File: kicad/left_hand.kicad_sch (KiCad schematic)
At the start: 29 parts, among them SW10 Gateron_ks_27, SW11 Gateron_ks_27, SW12 Gateron_ks_27, SW13 Gateron_ks_27, SW14 Gateron_ks_27, SW15 Gateron_ks_27, SW16 Gateron_ks_27, SW17 Gateron_ks_27, SW18 Gateron_ks_27, SW19 Gateron_ks_27, SW20 Gateron_ks_27, SW21 Gateron_ks_27, SW22 Gateron_ks_27, SW23 Gateron_ks_27, SW24 Gateron_ks_27, SW25 Gateron_ks_27, SW26 Gateron_ks_27, SW27 Gateron_ks_27, SW28 Gateron_ks_27, SW29 Gateron_ks_27, SW30 Gateron_ks_27, SW31 Gateron_ks_27, SW32 Gateron_ks_27, SW33 Gateron_ks_27, SW6 Gateron_ks_27, SW7 Gateron_ks_27, SW8 Gateron_ks_27, SW9 Gateron_ks_27, U2 74HC595

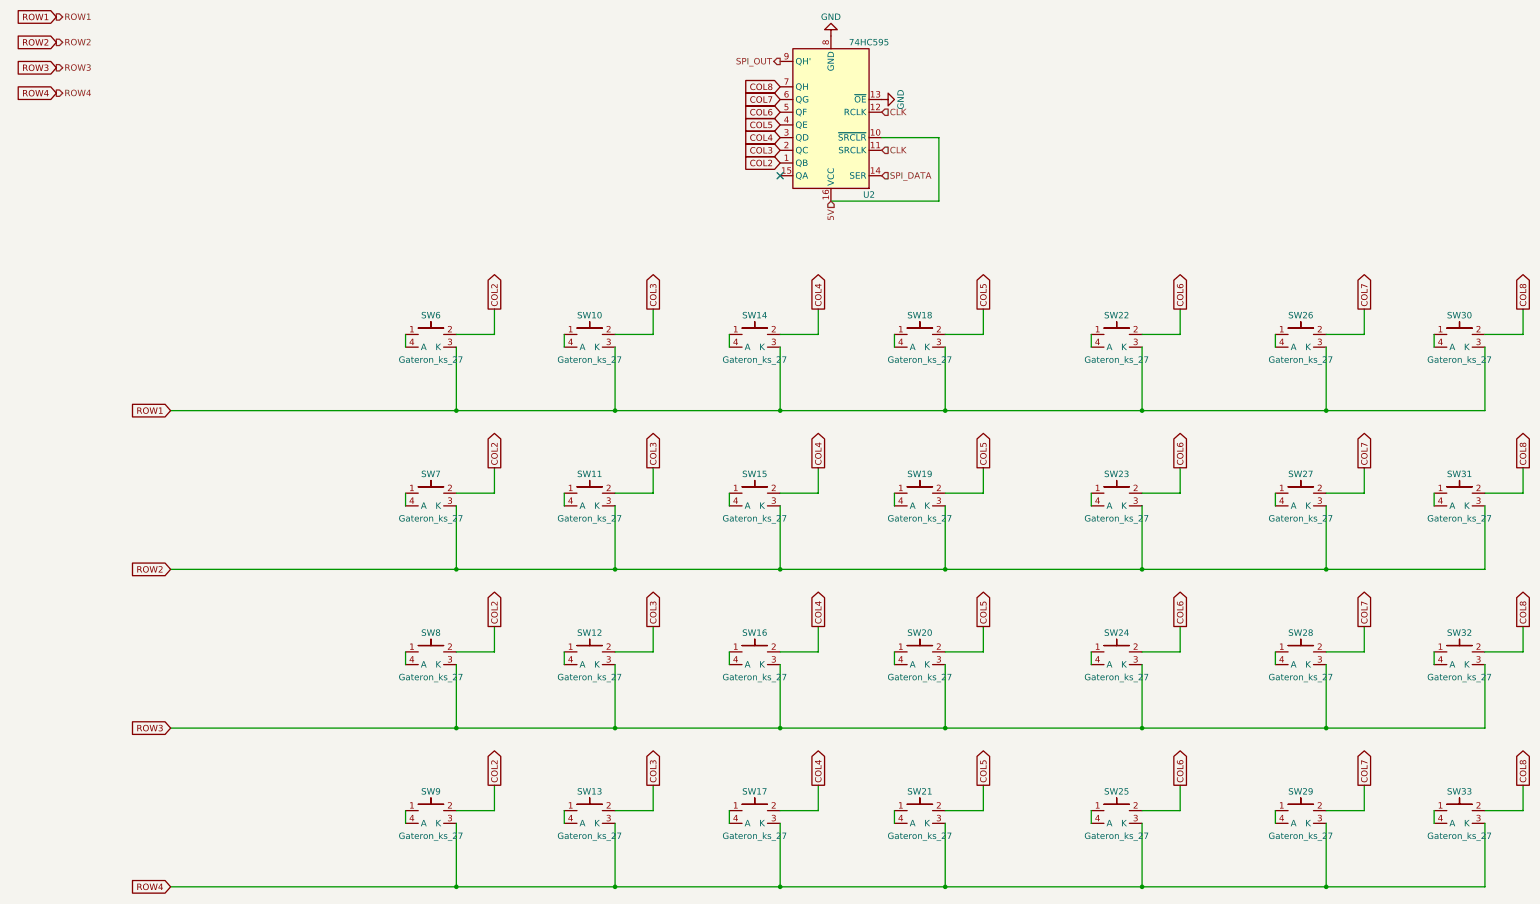
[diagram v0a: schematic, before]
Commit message: Last update
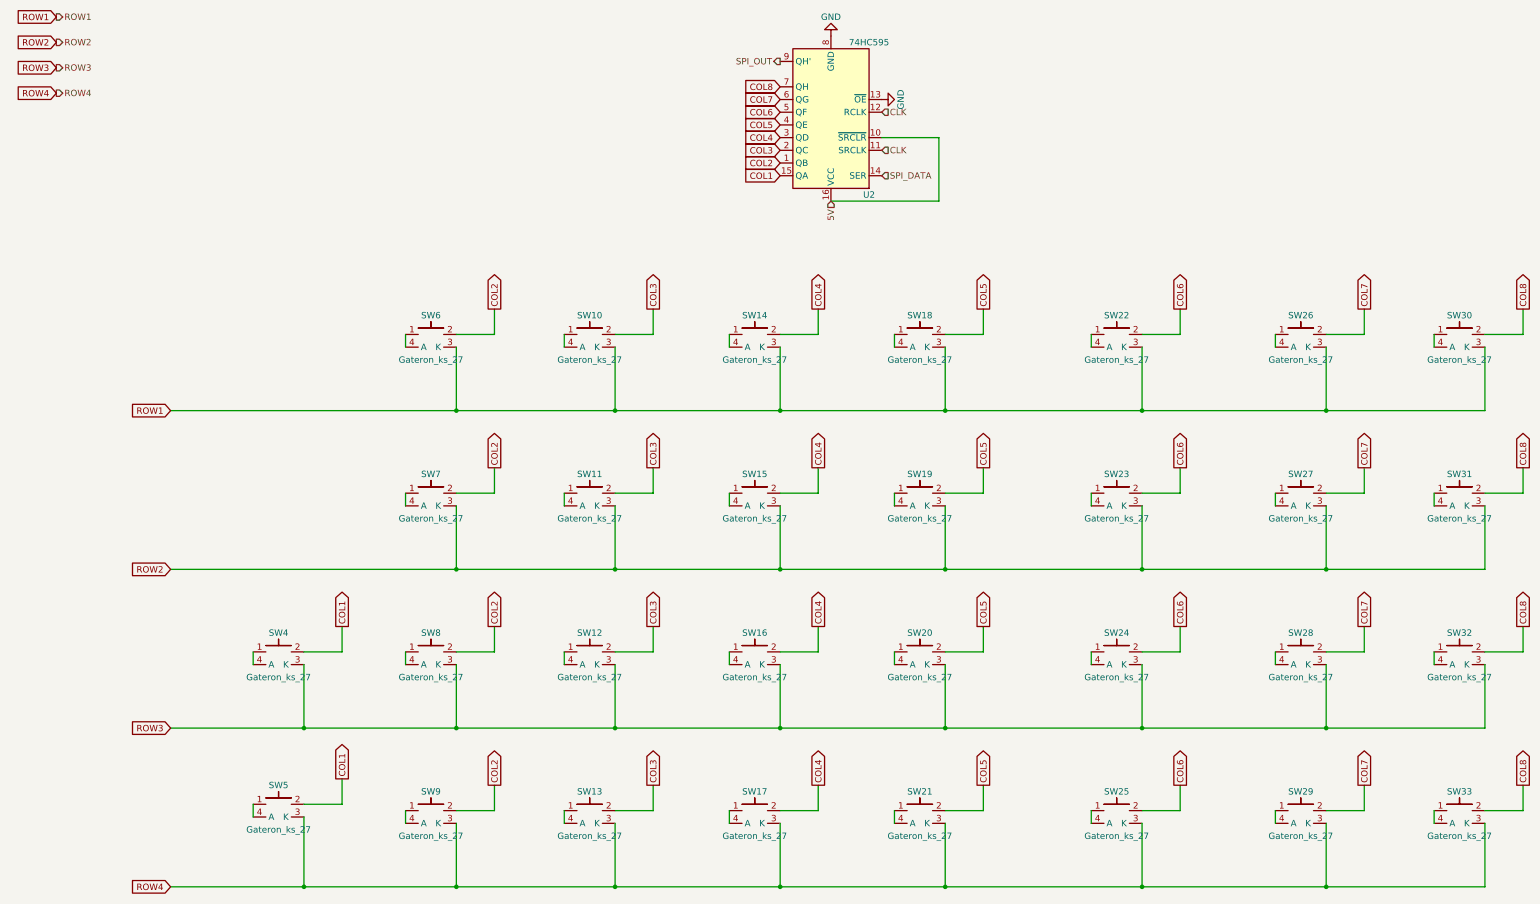
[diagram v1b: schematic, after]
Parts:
- added SW4, SW5: Gateron_ks_27, Keyboard:Gateron_ks_27, symbol keyboard:Gateron_ks_27
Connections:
- net ROW3: now also SW4.3 (K)
- net ROW4: now also SW5.3 (K)
- net COL1: now reaches U2.15 (QA)
- net COL1: now also SW4.2, SW5.2
- new net: SW5.1, SW5.4 (A)
- new net: SW4.1, SW4.4 (A)
- no-connect marks 1 -> 0
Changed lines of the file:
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@@
   (junction (at 182.88 163.83) (diameter 0) (color 0 0 0 0)
   )
+  (junction (at 87.63 227.33) (diameter 0) (color 0 0 0 0)
+  )
   (junction (at 215.9 132.08) (diameter 0) (color 0 0 0 0)
   )
@@
   (junction (at 292.1 227.33) (diameter 0) (color 0 0 0 0)
   )
+  (junction (at 87.63 195.58) (diameter 0) (color 0 0 0 0)
+  )
   (junction (at 215.9 227.33) (diameter 0) (color 0 0 0 0)
   )
@@
   (junction (at 118.11 195.58) (diameter 0) (color 0 0 0 0)
   )
-  (no_connect (at 182.88 85.09))
   (wire (pts (xy 149.86 227.33) (xy 118.11 227.33))
     (stroke (width 0) (type default) (color 0 0 0 0))
@@
     (stroke (width 0) (type default) (color 0 0 0 0))
   )
-  (wire (pts (xy 60.96 227.33) (xy 118.11 227.33))
+  (wire (pts (xy 60.96 227.33) (xy 87.63 227.33))
     (stroke (width 0) (type default) (color 0 0 0 0))
   )
@@
     (stroke (width 0) (type default) (color 0 0 0 0))
   )
+  (wire (pts (xy 87.63 180.34) (xy 95.25 180.34))
+    (stroke (width 0) (type default) (color 0 0 0 0))
+  )
   (wire (pts (xy 323.85 151.13) (xy 323.85 163.83))
     (stroke (width 0) (type default) (color 0 0 0 0))
@@
     (stroke (width 0) (type default) (color 0 0 0 0))
   )
+  (wire (pts (xy 77.47 180.34) (xy 77.47 182.88))
+    (stroke (width 0) (type default) (color 0 0 0 0))
+  )
   (wire (pts (xy 323.85 119.38) (xy 323.85 132.08))
     (stroke (width 0) (type default) (color 0 0 0 0))
@@
     (stroke (width 0) (type default) (color 0 0 0 0))
   )
+  (wire (pts (xy 87.63 195.58) (xy 118.11 195.58))
+    (stroke (width 0) (type default) (color 0 0 0 0))
+  )
   (wire (pts (xy 157.48 148.59) (xy 157.48 143.51))
     (stroke (width 0) (type default) (color 0 0 0 0))
@@
     (stroke (width 0) (type default) (color 0 0 0 0))
   )
+  (wire (pts (xy 87.63 182.88) (xy 87.63 195.58))
+    (stroke (width 0) (type default) (color 0 0 0 0))
+  )
   (wire (pts (xy 182.88 214.63) (xy 182.88 227.33))
     (stroke (width 0) (type default) (color 0 0 0 0))
@@
     (stroke (width 0) (type default) (color 0 0 0 0))
   )
+  (wire (pts (xy 77.47 210.82) (xy 77.47 213.36))
+    (stroke (width 0) (type default) (color 0 0 0 0))
+  )
   (wire (pts (xy 214.63 90.17) (xy 193.04 90.17))
     (stroke (width 0) (type default) (color 0 0 0 0))
@@
     (stroke (width 0) (type default) (color 0 0 0 0))
   )
-  (wire (pts (xy 60.96 195.58) (xy 118.11 195.58))
+  (wire (pts (xy 60.96 195.58) (xy 87.63 195.58))
     (stroke (width 0) (type default) (color 0 0 0 0))
   )
@@
     (stroke (width 0) (type default) (color 0 0 0 0))
   )
+  (wire (pts (xy 87.63 210.82) (xy 95.25 210.82))
+    (stroke (width 0) (type default) (color 0 0 0 0))
+  )
   (wire (pts (xy 149.86 163.83) (xy 182.88 163.83))
     (stroke (width 0) (type default) (color 0 0 0 0))
@@
     (stroke (width 0) (type default) (color 0 0 0 0))
   )
+  (wire (pts (xy 87.63 227.33) (xy 118.11 227.33))
+    (stroke (width 0) (type default) (color 0 0 0 0))
+  )
   (wire (pts (xy 125.73 116.84) (xy 125.73 111.76))
     (stroke (width 0) (type default) (color 0 0 0 0))
@@
     (stroke (width 0) (type default) (color 0 0 0 0))
   )
+  (wire (pts (xy 87.63 213.36) (xy 87.63 227.33))
+    (stroke (width 0) (type default) (color 0 0 0 0))
+  )
   (wire (pts (xy 172.72 148.59) (xy 172.72 151.13))
     (stroke (width 0) (type default) (color 0 0 0 0))
@@
     (stroke (width 0) (type default) (color 0 0 0 0))
   )
+  (wire (pts (xy 95.25 180.34) (xy 95.25 175.26))
+    (stroke (width 0) (type default) (color 0 0 0 0))
+  )
   (wire (pts (xy 299.72 212.09) (xy 299.72 207.01))
     (stroke (width 0) (type default) (color 0 0 0 0))
   )
+  (wire (pts (xy 95.25 210.82) (xy 95.25 205.74))
+    (stroke (width 0) (type default) (color 0 0 0 0))
+  )
   (wire (pts (xy 223.52 180.34) (xy 223.52 175.26))
     (stroke (width 0) (type default) (color 0 0 0 0))
@@
     )
   )
+  (global_label "COL1" (shape output) (at 95.25 175.26 90) (fields_autoplaced)
+    (effects (font (size 1.27 1.27)) (justify left))
+    (property "Intersheet References" "${INTERSHEET_REFS}" (id 0) (at 95.1706 168.0088 90)
+      (effects (font (size 1.27 1.27)) (justify left) hide)
+    )
+  )
   (global_label "COL3" (shape output) (at 157.48 111.76 90) (fields_autoplaced)
     (effects (font (size 1.27 1.27)) (justify left))
@@
     )
   )
+  (global_label "COL1" (shape output) (at 95.25 205.74 90) (fields_autoplaced)
+    (effects (font (size 1.27 1.27)) (justify left))
+    (property "Intersheet References" "${INTERSHEET_REFS}" (id 0) (at 95.1706 198.4888 90)
+      (effects (font (size 1.27 1.27)) (justify left) hide)
+    )
+  )
   (global_label "ROW1" (shape input) (at 60.96 132.08 180) (fields_autoplaced)
     (effects (font (size 1.27 1.27)) (justify right))
@@
     (property "Intersheet References" "${INTERSHEET_REFS}" (id 0) (at 157.4006 136.2588 90)
       (effects (font (size 1.27 1.27)) (justify left) hide)
+    )
+  )
+  (global_label "COL1" (shape input) (at 182.88 85.09 180) (fields_autoplaced)
+    (effects (font (size 1.27 1.27)) (justify right))
+    (property "Intersheet References" "${INTERSHEET_REFS}" (id 0) (at 175.6288 85.0106 0)
+      (effects (font (size 1.27 1.27)) (justify right) hide)
     )
   )
@@
     (pin "4")
   )
+  (symbol (lib_id "keyboard:Gateron_ks_27") (at 77.47 210.82 0) (unit 1)
+    (in_bom yes) (on_board yes)
+    (property "Reference" "SW5" (id 0) (at 82.55 207.01 0))
+    (property "Value" "Gateron_ks_27" (id 1) (at 82.55 215.9 0))
+    (property "Footprint" "Keyboard:Gateron_ks_27" (id 2) (at 77.47 210.82 0)
+      (effects (font (size 1.27 1.27)) hide)
+    )
+    (property "Datasheet" "" (id 3) (at 77.47 210.82 0)
+      (effects (font (size 1.27 1.27)) hide)
+    )
+    (pin "1")
+    (pin "2")
+    (pin "3")
+    (pin "4")
+  )
   (symbol (lib_id "keyboard:Gateron_ks_27") (at 313.69 116.84 0) (unit 1)
     (in_bom yes) (on_board yes)
@@
       (effects (font (size 1.27 1.27)) hide)
     )
+    (pin "1")
+    (pin "2")
+    (pin "3")
+    (pin "4")
+  )
+  (symbol (lib_id "keyboard:Gateron_ks_27") (at 77.47 180.34 0) (unit 1)
+    (in_bom yes) (on_board yes)
+    (property "Reference" "SW4" (id 0) (at 82.55 176.53 0))
+    (property "Value" "Gateron_ks_27" (id 1) (at 82.55 185.42 0))
+    (property "Footprint" "Keyboard:Gateron_ks_27" (id 2) (at 77.47 180.34 0)
+      (effects (font (size 1.27 1.27)) hide)
+    )
+    (property "Datasheet" "" (id 3) (at 77.47 180.34 0)
+      (effects (font (size 1.27 1.27)) hide)
+    )
